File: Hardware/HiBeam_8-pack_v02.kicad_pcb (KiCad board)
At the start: 2 copper layers, 28.4 x 28.4 mm, 38 parts, among them J1 M01PTH, J2 M01PTH, J3 M01PTH, J4 M01PTH, J5 M01PTH, J6 M01PTH, J7 M01PTH, J8 M01PTH, U1 APA102, U2 APA102, U3 APA102, U4 APA102, U5 APA102, U6 APA102, U7 APA102, U8 APA102

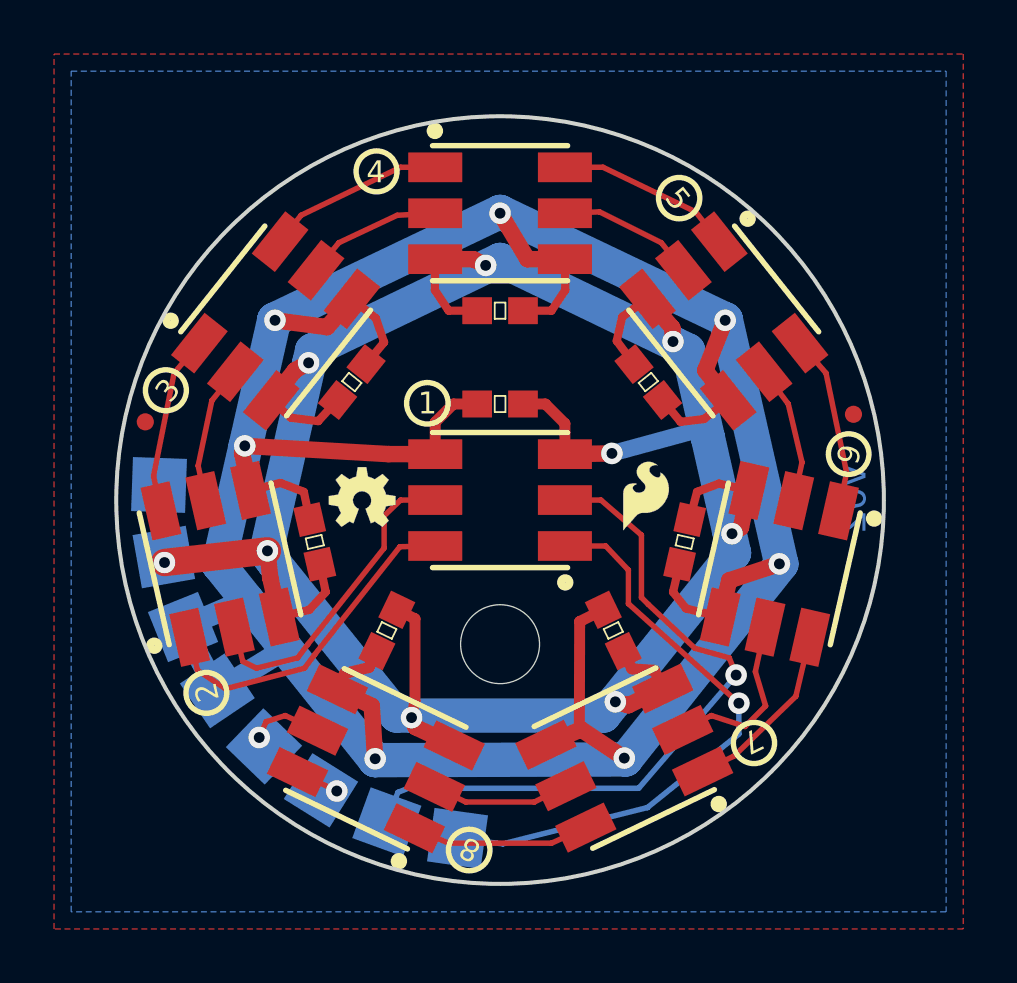
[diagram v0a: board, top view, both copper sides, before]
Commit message: Silk fixes.
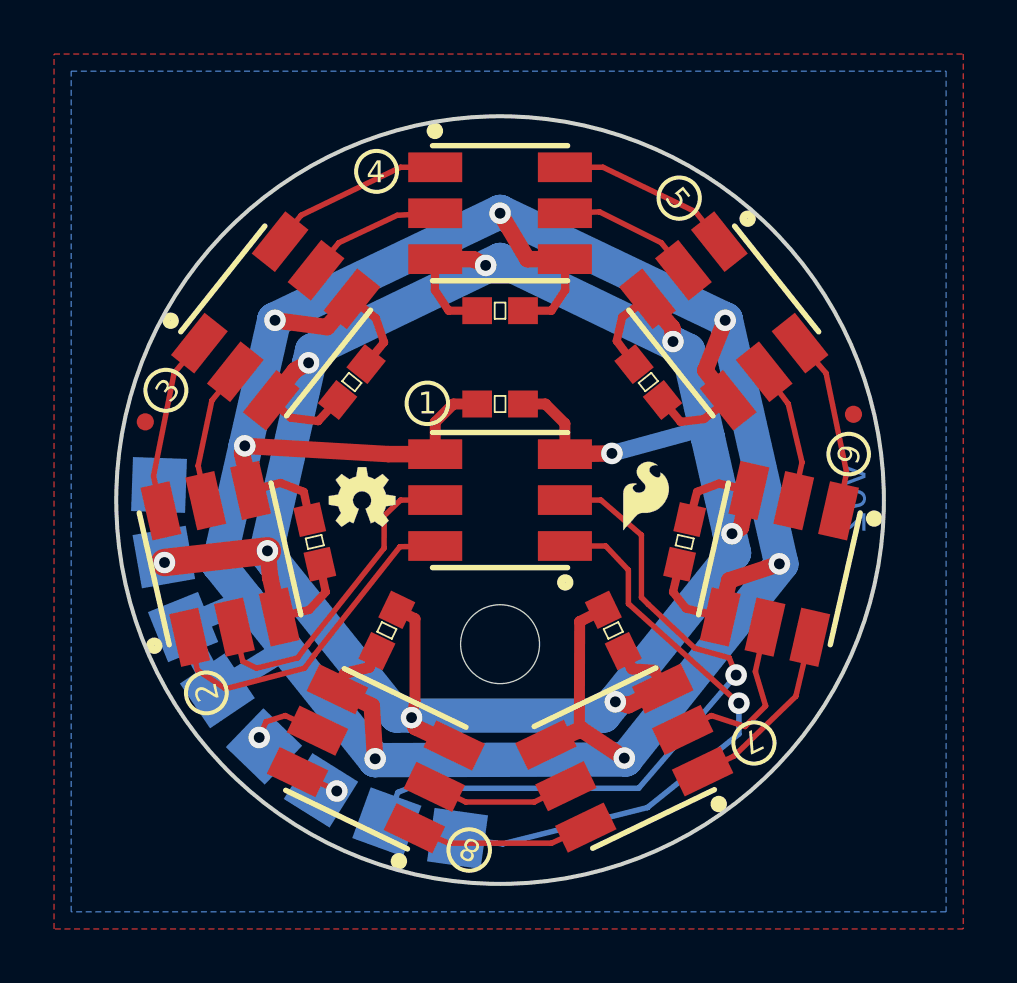
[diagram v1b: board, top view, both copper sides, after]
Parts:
- moved ? 2.11 mm to (152.5, 91.9)
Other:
- rule pad_to_mask_clearance: 0.2 -> 0.1016
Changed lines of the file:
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@@
     (area 121.641205 72.114999 273.4474 194.4604)
     (thickness 1.6)
-    (drawings 40)
+    (drawings 39)
     (tracks 241)
     (zones 0)
@@
   (layers
     (0 F.Cu signal)
-    (31 B.Cu signal hide)
-    (32 B.Adhes user)
+    (31 B.Cu signal)
+    (32 B.Adhes user hide)
     (33 F.Adhes user hide)
-    (34 B.Paste user)
-    (35 F.Paste user)
-    (36 B.SilkS user hide)
+    (34 B.Paste user hide)
+    (35 F.Paste user hide)
+    (36 B.SilkS user)
     (37 F.SilkS user)
-    (38 B.Mask user)
+    (38 B.Mask user hide)
     (39 F.Mask user)
     (40 Dwgs.User user)
-    (41 Cmts.User user)
-    (42 Eco1.User user)
-    (43 Eco2.User user)
+    (41 Cmts.User user hide)
+    (42 Eco1.User user hide)
+    (43 Eco2.User user hide)
     (44 Edge.Cuts user)
-    (45 Margin user)
+    (45 Margin user hide)
     (46 B.CrtYd user hide)
     (47 F.CrtYd user hide)
-    (48 B.Fab user)
-    (49 F.Fab user)
+    (48 B.Fab user hide)
+    (49 F.Fab user hide)
   )
   (setup
@@
     (pad_size 1.524 1.524)
     (pad_drill 0.762)
-    (pad_to_mask_clearance 0.2)
+    (pad_to_mask_clearance 0.1016)
     (aux_axis_origin 0 0)
-    (visible_elements FFF8FF7F)
+    (visible_elements FFF9FF7F)
     (pcbplotparams
-      (layerselection 0x000fc_ffffffff)
+      (layerselection 0x010fc_ffffffff)
       (usegerberextensions false)
       (excludeedgelayer true)
@@
   )
   (module SparkFun:SFE_LOGO_NAME_FLAME_.1 (layer B.Cu)
-    (at 152.5524 93.98 180)
+    (at 152.5016 91.8718 180)
     (descr "SPARKFUN FONT LOGO W/ FLAME - 0.1\" HEIGHT - SILKSCREEN")
     (tags "SPARKFUN FONT LOGO W/ FLAME - 0.1\" HEIGHT - SILKSCREEN")
@@
       (net 2 GND))
   )
-  (gr_circle (center 145.542 110.744) (end 146.177 111.1758) (layer F.SilkS) (width 0.2))
-  (gr_circle (center 142.113 85.6234) (end 142.6972 86.106) (layer F.SilkS) (width 0.2))
-  (gr_circle (center 153.3144 86.614) (end 154.0256 86.8934) (layer F.SilkS) (width 0.2))
-  (gr_circle (center 156.083 106.7816) (end 156.7434 107.1626) (layer F.SilkS) (width 0.2))
-  (gr_circle (center 159.5882 96.0882) (end 160.274 96.393) (layer F.SilkS) (width 0.2))
-  (gr_circle (center 135.8138 104.9274) (end 136.3218 105.4862) (layer F.SilkS) (width 0.2))
-  (gr_circle (center 143.9926 94.2086) (end 144.6276 94.6404) (layer F.SilkS) (width 0.2))
-  (gr_circle (center 134.3152 93.726) (end 134.8994 94.2086) (layer F.SilkS) (width 0.2))
+  (gr_circle (center 145.542 110.744) (end 146.177 111.1758) (layer F.SilkS) (width 0.15))
+  (gr_circle (center 142.113 85.6234) (end 142.6972 86.106) (layer F.SilkS) (width 0.15))
+  (gr_circle (center 153.3144 86.614) (end 154.0256 86.8934) (layer F.SilkS) (width 0.15))
+  (gr_circle (center 156.083 106.7816) (end 156.7434 107.1626) (layer F.SilkS) (width 0.15))
+  (gr_circle (center 159.5882 96.0882) (end 160.274 96.393) (layer F.SilkS) (width 0.15))
+  (gr_circle (center 135.8138 104.9274) (end 136.3218 105.4862) (layer F.SilkS) (width 0.15))
+  (gr_circle (center 143.9926 94.2086) (end 144.6276 94.6404) (layer F.SilkS) (width 0.15))
+  (gr_circle (center 134.3152 93.726) (end 134.8994 94.2086) (layer F.SilkS) (width 0.15))
   (gr_text 8 (at 145.5674 110.7186 154.3) (layer F.SilkS)
     (effects (font (size 0.8128 0.8128) (thickness 0.1778)))
@@
     (effects (font (size 1.016 1.016) (thickness 0.2032)) (justify mirror))
   )
-  (gr_text "HiBeams 8-pack" (at 146.685 94.615) (layer B.SilkS)
-    (effects (font (size 1.016 1.016) (thickness 0.2032)) (justify mirror))
+  (gr_text "HiBeams 8-pack" (at 146.685 92.6592) (layer B.SilkS)
+    (effects (font (size 1.5 1.5) (thickness 0.3)) (justify mirror))
   )
   (gr_text v02 (at 159.7406 97.7646 90) (layer B.Cu)
@@
   (gr_circle (center 146.685 97.79) (end 157.226 107.315) (layer Edge.Cuts) (width 0.15))
   (gr_circle (center 146.685 97.79) (end 149.479 105.41) (layer Dwgs.User) (width 0.2))
-  (target plus (at 146.685 97.79) (size 5) (width 0.15) (layer Edge.Cuts))
   (segment (start 149.619135 106.301539) (end 149.6314 102.2858) (width 0.4064) (layer F.Cu) (net 1))
   (segment (start 149.6314 102.2858) (end 150.508101 101.851562) (width 0.4064) (layer F.Cu) (net 1))
